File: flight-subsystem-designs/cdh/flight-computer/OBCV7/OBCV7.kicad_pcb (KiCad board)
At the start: 4 copper layers, 90.3 x 95.9 mm, 45 parts, among them U1 BEAGLEBONEBLACK, U3 TCAN337G, U4 MCP7940N-xSN, U5 ADM3485EARZ, U6 MAX706RESA+T, U7 TMP36xS

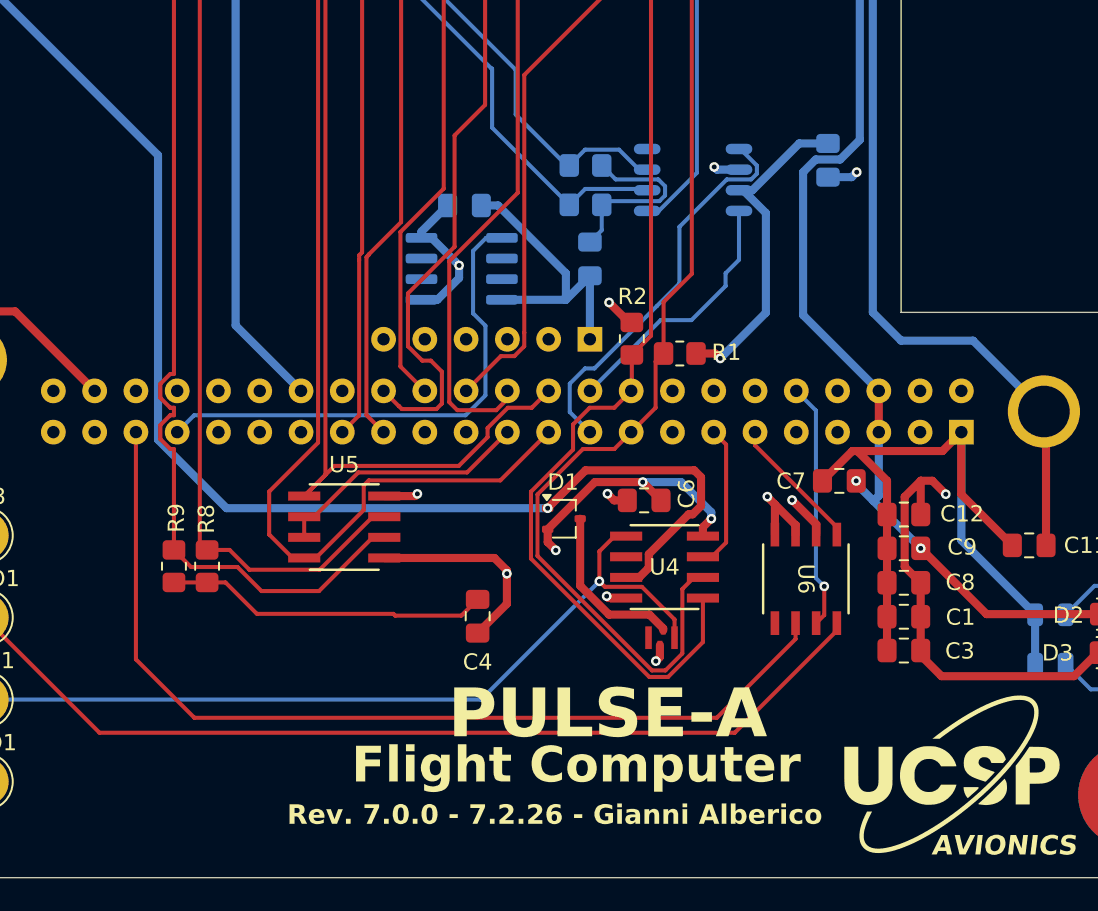
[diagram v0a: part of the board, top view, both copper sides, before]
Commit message: Perhaps technology is hubris manifest
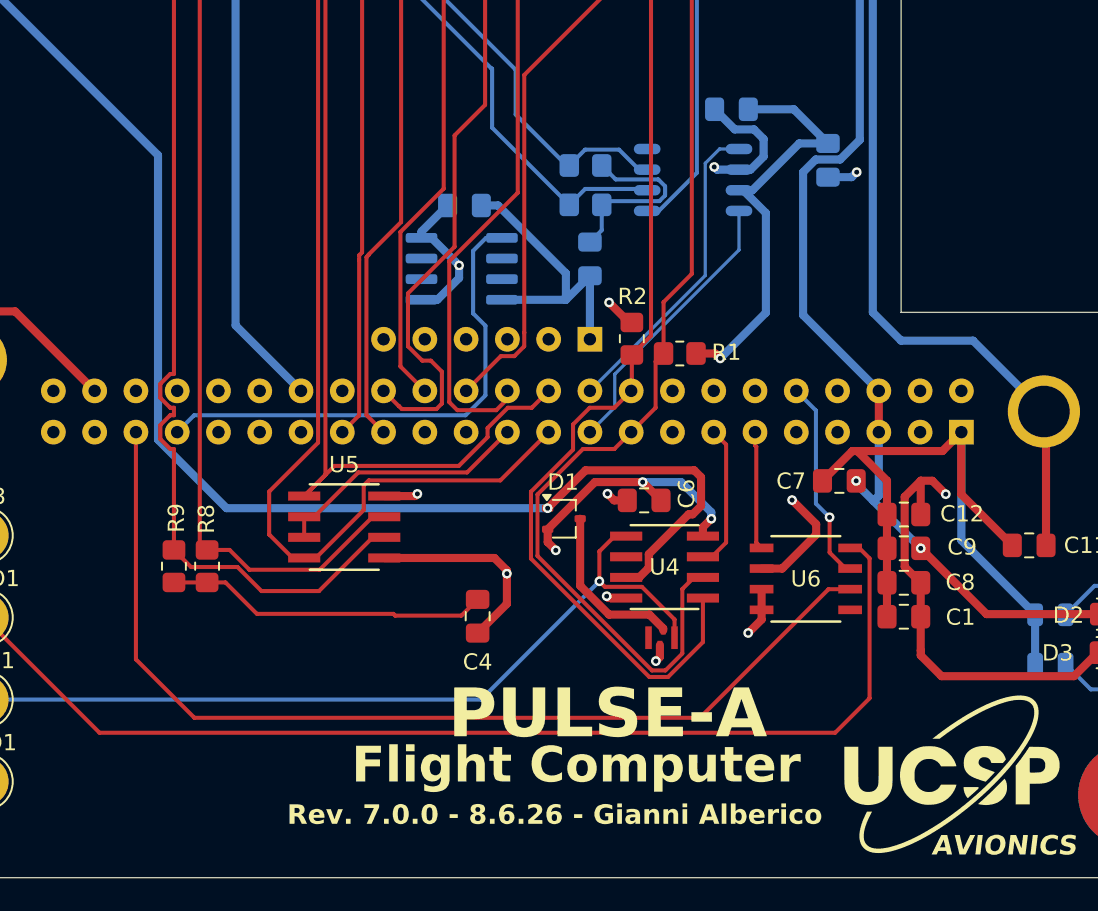
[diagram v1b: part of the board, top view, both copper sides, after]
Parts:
- C3: moved to B.Cu
- C5: value 10nF -> 5nF
- moved C3 35.0 mm to (153.3, 79.0)
- turned U6 to 0 degrees
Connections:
- U1 pad P9_19: /DCAN1TX -> /DCAN0RX
- U1 pad P9_20: /DCAN1RX -> /DCAN0TX
- U3 pad 1: /DCAN1TX -> /DCAN0TX
- U3 pad 4: /DCAN1RX -> /DCAN0RX
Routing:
- net /DCAN1TX: track 24.4 -> 0.00 mm
- net /DCAN0TX: track 0.00 -> 19.4 mm
- net /DCAN0RX: track 0.00 -> 17.4 mm
- net /DCAN1RX: track 16.0 -> 0.00 mm
- net /3V3: track 81.1 -> 91.1 mm
- net Net-(U6-*WDO): track 58.5 -> 68.4 mm
- net /GPIO3_20: track 59.1 -> 62.7 mm
- net GND: track 145.9 -> 148.6 mm
- net /SYSRST: track 15.2 -> 12.5 mm
- net /MRV: track 8.39 -> 7.29 mm
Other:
- board text added: "Rev. 7.0.0 - 8.6.26 - Gianni Alberico"
- board text removed: "Rev. 7.0.0 - 7.2.26 - Gianni Alberico"
